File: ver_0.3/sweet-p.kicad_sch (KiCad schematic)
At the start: 50 parts, among them J1 Screw_Terminal_01x02, J2 Conn_01x11_Female, J3 Screw_Terminal_01x03, J4 Conn_01x08_Female, J5 Conn_01x06_Female, J6 Screw_Terminal_01x04, J7 Micro_SD_Card, U1 adafruit_tpl511x, U2 MCP1700-3302E_TO, U3 adafruit_ads1115, U4 ssd1306, U5 RFM95W-868S2, U6 Adafruit-Mini-GPS, U7 ds3231

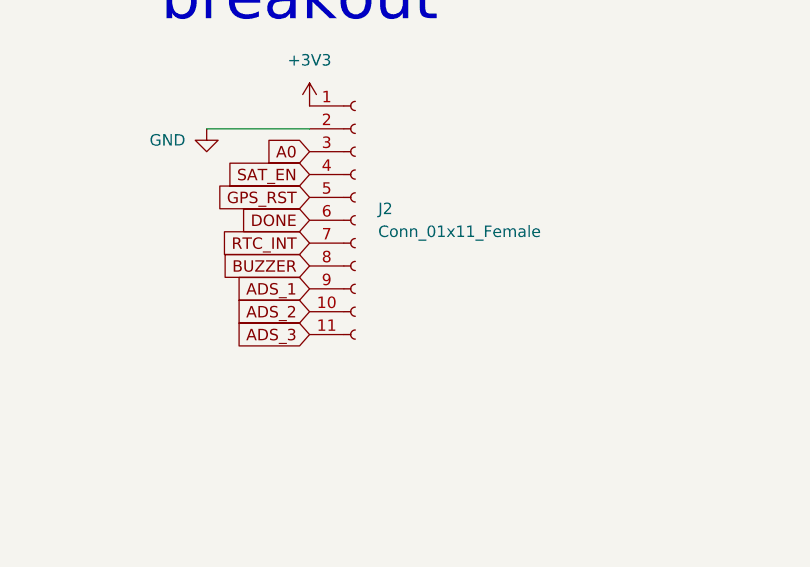
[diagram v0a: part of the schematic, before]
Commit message: fixed breakout
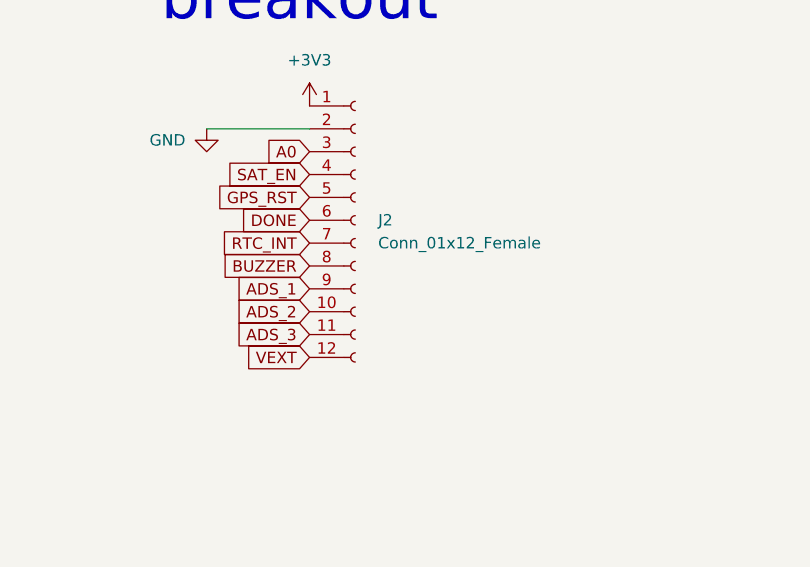
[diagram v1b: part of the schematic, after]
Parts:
- removed J2: Conn_01x11_Female, Connector_PinSocket_2.54mm:PinSocket_1x11_P2.54mm_Vertical, symbol Connector:Conn_01x11_Female
- added J2: Conn_01x12_Female, Connector_PinSocket_2.54mm:PinSocket_2x06_P2.54mm_Vertical, symbol Connector:Conn_01x12_Female
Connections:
- net +3V3: now also J2.1 (Pin_1)
- net A0: now also J2.3 (Pin_3)
- net ADS_1: now also J2.9 (Pin_9)
- net ADS_2: now also J2.10 (Pin_10)
- net ADS_3: now also J2.11 (Pin_11)
- net BUZZER: now also J2.8 (Pin_8)
- net DONE: now also J2.6 (Pin_6)
- net GND: now also J2.2 (Pin_2)
- net GPS_RST: now also J2.5 (Pin_5)
- net RTC_INT: now also J2.7 (Pin_7)
- net SAT_EN: now also J2.4 (Pin_4)
- net VEXT: now also J2.12 (Pin_12)

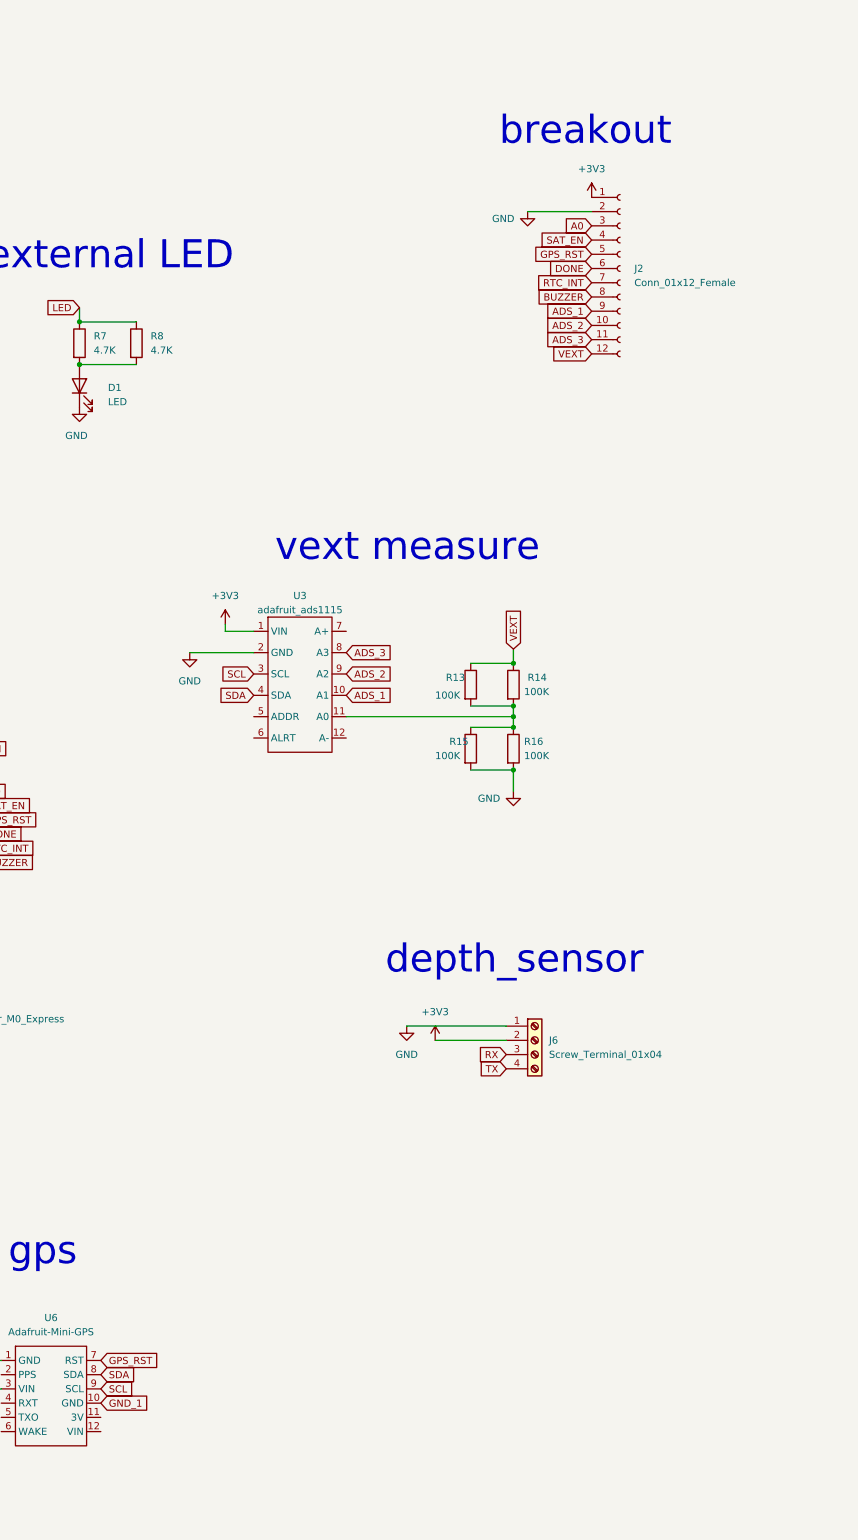
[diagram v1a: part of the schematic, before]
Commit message: update
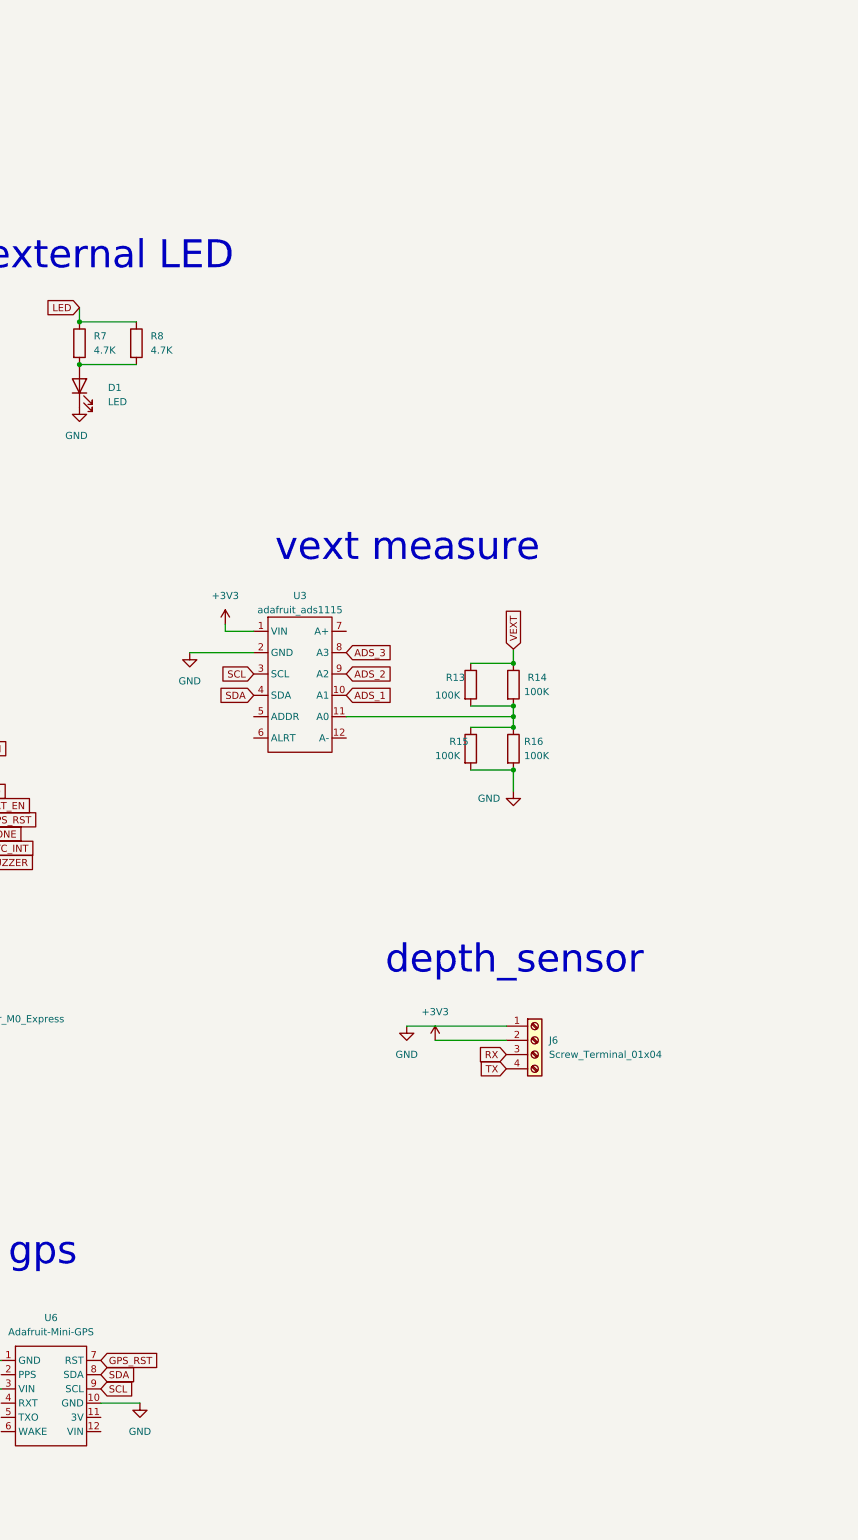
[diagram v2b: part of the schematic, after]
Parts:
- removed J2: Conn_01x12_Female, Connector_PinSocket_2.54mm:PinSocket_2x06_P2.54mm_Vertical, symbol Connector:Conn_01x12_Female
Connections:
- net GND_1 is gone; now on net GND: U6.10 (GND)
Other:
- note removed: "breakout"
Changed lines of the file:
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@@
+    (stroke (width 0) (type default) (color 0 0 0 0))
+  )
+  (wire (pts (xy -132.08 138.43) (xy -125.095 138.43))
     (stroke (width 0) (type default) (color 0 0 0 0))
   )
@@
     (stroke (width 0) (type default) (color 0 0 0 0))
   )
-  (wire (pts (xy -55.88 -74.295) (xy -44.45 -74.295))
-    (stroke (width 0) (type default) (color 0 0 0 0))
-  )
   (wire (pts (xy -143.51 -124.46) (xy -123.825 -124.46))
     (stroke (width 0) (type default) (color 0 0 0 0))
@@
     (effects (font (size 5 5)) (justify left bottom))
   )
-  (text "breakout" (at -60.96 -85.725 0)
-    (effects (font (size 5 5)) (justify left bottom))
-  )
   (text "ssd1306" (at 33.02 100.33 0)
     (effects (font (size 1.27 1.27)) (justify left bottom))
@@
     )
   )
-  (global_label "VEXT" (shape input) (at -44.45 -48.895 180) (fields_autoplaced)
-    (effects (font (size 1.27 1.27)) (justify right))
-    (property "Intersheet References" "${INTERSHEET_REFS}" (id 0) (at -51.2779 -48.9744 0)
-      (effects (font (size 1.27 1.27)) (justify right) hide)
-    )
-  )
   (global_label "SAT_EN" (shape input) (at -261.62 30.48 0) (fields_autoplaced)
     (effects (font (size 1.27 1.27)) (justify left))
@@
     )
   )
-  (global_label "GND_1" (shape input) (at -132.08 138.43 0) (fields_autoplaced)
-    (effects (font (size 1.27 1.27)) (justify left))
-    (property "Intersheet References" "${INTERSHEET_REFS}" (id 0) (at -123.6193 138.3506 0)
-      (effects (font (size 1.27 1.27)) (justify left) hide)
-    )
-  )
   (global_label "SCL" (shape input) (at 45.72 114.3 0) (fields_autoplaced)
     (effects (font (size 1.27 1.27)) (justify left))
@@
     )
   )
-  (global_label "ADS_2" (shape input) (at -44.45 -53.975 180) (fields_autoplaced)
-    (effects (font (size 1.27 1.27)) (justify right))
-    (property "Intersheet References" "${INTERSHEET_REFS}" (id 0) (at -52.6083 -53.8956 0)
-      (effects (font (size 1.27 1.27)) (justify right) hide)
-    )
-  )
   (global_label "VEXT" (shape input) (at -58.42 3.81 90) (fields_autoplaced)
     (effects (font (size 1.27 1.27)) (justify left))
@@
     )
   )
-  (global_label "A0" (shape input) (at -44.45 -71.755 180) (fields_autoplaced)
-    (effects (font (size 1.27 1.27)) (justify right))
-    (property "Intersheet References" "${INTERSHEET_REFS}" (id 0) (at -49.1612 -71.6756 0)
-      (effects (font (size 1.27 1.27)) (justify right) hide)
-    )
-  )
   (global_label "RTC_INT" (shape input) (at 77.47 180.34 0) (fields_autoplaced)
     (effects (font (size 1.27 1.27)) (justify left))
@@
     )
   )
-  (global_label "ADS_1" (shape input) (at -44.45 -56.515 180) (fields_autoplaced)
-    (effects (font (size 1.27 1.27)) (justify right))
-    (property "Intersheet References" "${INTERSHEET_REFS}" (id 0) (at -52.6083 -56.4356 0)
-      (effects (font (size 1.27 1.27)) (justify right) hide)
-    )
-  )
   (global_label "DONE" (shape input) (at -77.47 -124.46 0) (fields_autoplaced)
     (effects (font (size 1.27 1.27)) (justify left))
@@
     )
   )
-  (global_label "GPS_RST" (shape input) (at -44.45 -66.675 180) (fields_autoplaced)
-    (effects (font (size 1.27 1.27)) (justify right))
-    (property "Intersheet References" "${INTERSHEET_REFS}" (id 0) (at -55.0274 -66.5956 0)
-      (effects (font (size 1.27 1.27)) (justify right) hide)
-    )
-  )
   (global_label "ADS_2" (shape input) (at -88.265 8.255 0) (fields_autoplaced)
     (effects (font (size 1.27 1.27)) (justify left))
@@
     )
   )
-  (global_label "DONE" (shape input) (at -44.45 -64.135 180) (fields_autoplaced)
-    (effects (font (size 1.27 1.27)) (justify right))
-    (property "Intersheet References" "${INTERSHEET_REFS}" (id 0) (at -51.9431 -64.0556 0)
-      (effects (font (size 1.27 1.27)) (justify right) hide)
-    )
-  )
   (global_label "RX" (shape input) (at -59.69 76.2 180) (fields_autoplaced)
     (effects (font (size 1.27 1.27)) (justify right))
@@
     )
   )
-  (global_label "ADS_3" (shape input) (at -44.45 -51.435 180) (fields_autoplaced)
-    (effects (font (size 1.27 1.27)) (justify right))
-    (property "Intersheet References" "${INTERSHEET_REFS}" (id 0) (at -52.6083 -51.3556 0)
-      (effects (font (size 1.27 1.27)) (justify right) hide)
-    )
-  )
   (global_label "SDA" (shape input) (at 45.72 118.11 0) (fields_autoplaced)
     (effects (font (size 1.27 1.27)) (justify left))
@@
     )
   )
-  (global_label "BUZZER" (shape input) (at -44.45 -59.055 180) (fields_autoplaced)
-    (effects (font (size 1.27 1.27)) (justify right))
-    (property "Intersheet References" "${INTERSHEET_REFS}" (id 0) (at -54.3017 -58.9756 0)
-      (effects (font (size 1.27 1.27)) (justify right) hide)
-    )
-  )
   (global_label "SDA" (shape input) (at 44.45 187.96 180) (fields_autoplaced)
     (effects (font (size 1.27 1.27)) (justify right))
     (property "Intersheet References" "${INTERSHEET_REFS}" (id 0) (at 38.4688 187.8806 0)
-      (effects (font (size 1.27 1.27)) (justify right) hide)
-    )
-  )
-  (global_label "RTC_INT" (shape input) (at -44.45 -61.595 180) (fields_autoplaced)
-    (effects (font (size 1.27 1.27)) (justify right))
-    (property "Intersheet References" "${INTERSHEET_REFS}" (id 0) (at -54.2412 -61.5156 0)
-      (effects (font (size 1.27 1.27)) (justify right) hide)
-    )
-  )
-  (global_label "SAT_EN" (shape input) (at -44.45 -69.215 180) (fields_autoplaced)
-    (effects (font (size 1.27 1.27)) (justify right))
-    (property "Intersheet References" "${INTERSHEET_REFS}" (id 0) (at -53.576 -69.1356 0)
       (effects (font (size 1.27 1.27)) (justify right) hide)
     )
@@
     (pin "1")
   )
-  (symbol (lib_id "power:+3V3") (at -44.45 -76.835 0) (unit 1)
-    (in_bom yes) (on_board yes) (fields_autoplaced)
-    (property "Reference" "#PWR07" (id 0) (at -44.45 -73.025 0)
-      (effects (font (size 1.27 1.27)) hide)
-    )
-    (property "Value" "+3V3" (id 1) (at -44.45 -81.915 0))
-    (property "Footprint" "" (id 2) (at -44.45 -76.835 0)
-      (effects (font (size 1.27 1.27)) hide)
-    )
-    (property "Datasheet" "" (id 3) (at -44.45 -76.835 0)
-      (effects (font (size 1.27 1.27)) hide)
-    )
-    (pin "1")
-  )
   (symbol (lib_id "sweet-p:adafruit_tpl511x") (at -86.36 -133.35 0) (unit 1)
     (in_bom yes) (on_board yes) (fields_autoplaced)
@@
     (pin "1")
   )
-  (symbol (lib_id "power:GND") (at -55.88 -74.295 0) (unit 1)
-    (in_bom yes) (on_board yes)
-    (property "Reference" "#PWR08" (id 0) (at -55.88 -67.945 0)
-      (effects (font (size 1.27 1.27)) hide)
-    )
-    (property "Value" "GND" (id 1) (at -62.23 -73.025 0)
-      (effects (font (size 1.27 1.27)) (justify left))
-    )
-    (property "Footprint" "" (id 2) (at -55.88 -74.295 0)
-      (effects (font (size 1.27 1.27)) hide)
-    )
-    (property "Datasheet" "" (id 3) (at -55.88 -74.295 0)
+  (symbol (lib_id "power:GND") (at -125.095 138.43 0) (unit 1)
+    (in_bom yes) (on_board yes) (fields_autoplaced)
+    (property "Reference" "#PWR?" (id 0) (at -125.095 144.78 0)
+      (effects (font (size 1.27 1.27)) hide)
+    )
+    (property "Value" "GND" (id 1) (at -125.095 143.51 0))
+    (property "Footprint" "" (id 2) (at -125.095 138.43 0)
+      (effects (font (size 1.27 1.27)) hide)
+    )
+    (property "Datasheet" "" (id 3) (at -125.095 138.43 0)
       (effects (font (size 1.27 1.27)) hide)
     )
@@
     (pin "1")
   )
-  (symbol (lib_id "Connector:Conn_01x12_Female") (at -39.37 -64.135 0) (unit 1)
-    (in_bom yes) (on_board yes) (fields_autoplaced)
-    (property "Reference" "J2" (id 0) (at -36.83 -64.1351 0)
-      (effects (font (size 1.27 1.27)) (justify left))
-    )
-    (property "Value" "Conn_01x12_Female" (id 1) (at -36.83 -61.5951 0)
-      (effects (font (size 1.27 1.27)) (justify left))
-    )
-    (property "Footprint" "Connector_PinSocket_2.54mm:PinSocket_2x06_P2.54mm_Vertical" (id 2) (at -39.37 -64.135 0)
-      (effects (font (size 1.27 1.27)) hide)
-    )
-    (property "Datasheet" "~" (id 3) (at -39.37 -64.135 0)
-      (effects (font (size 1.27 1.27)) hide)
-    )
-    (pin "1")
-    (pin "10")
-    (pin "11")
-    (pin "12")
-    (pin "2")
-    (pin "3")
-    (pin "4")
-    (pin "5")
-    (pin "6")
-    (pin "7")
-    (pin "8")
-    (pin "9")
-  )
   (symbol (lib_id "Device:R") (at -125.73 -50.8 0) (unit 1)
     (in_bom yes) (on_board yes) (fields_autoplaced)
@@
       (reference "#PWR06") (unit 1) (value "GND") (footprint "")
     )
-    (path "/80b1e8b0-c14a-43f3-8c02-df696b45978a"
-      (reference "#PWR07") (unit 1) (value "+3V3") (footprint "")
-    )
-    (path "/cba62e84-41d5-4142-a06a-c47b4bef012c"
-      (reference "#PWR08") (unit 1) (value "GND") (footprint "")
-    )
     (path "/edd9ae1f-b214-4924-bbe9-6791b913da4c"
       (reference "#PWR09") (unit 1) (value "+3V3") (footprint "")
@@
       (reference "#PWR043") (unit 1) (value "GND") (footprint "")
     )
+    (path "/d7a87d32-960d-4b6c-9ec6-e9cc6793a0ff"
+      (reference "#PWR?") (unit 1) (value "GND") (footprint "")
+    )
     (path "/183fe64b-877b-44e3-91b5-dd0a6ba3e1e1"
       (reference "A1") (unit 1) (value "Adafruit_Feather_M0_Express") (footprint "Module:Adafruit_Feather")
@@
       (reference "J1") (unit 1) (value "Screw_Terminal_01x02") (footprint "TerminalBlock_Phoenix:TerminalBlock_Phoenix_PT-1,5-2-5.0-H_1x02_P5.00mm_Horizontal")
     )
-    (path "/f1f261cd-aaf9-4dd2-beec-91fdb571c969"
-      (reference "J2") (unit 1) (value "Conn_01x12_Female") (footprint "Connector_PinSocket_2.54mm:PinSocket_2x06_P2.54mm_Vertical")
-    )
     (path "/356a682b-39b5-417e-8373-9ae81bd97f29"
